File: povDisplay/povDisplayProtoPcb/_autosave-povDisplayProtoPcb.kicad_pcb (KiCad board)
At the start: 4 copper layers, 41 parts, among them J5 Conn_02x06_Odd_Even

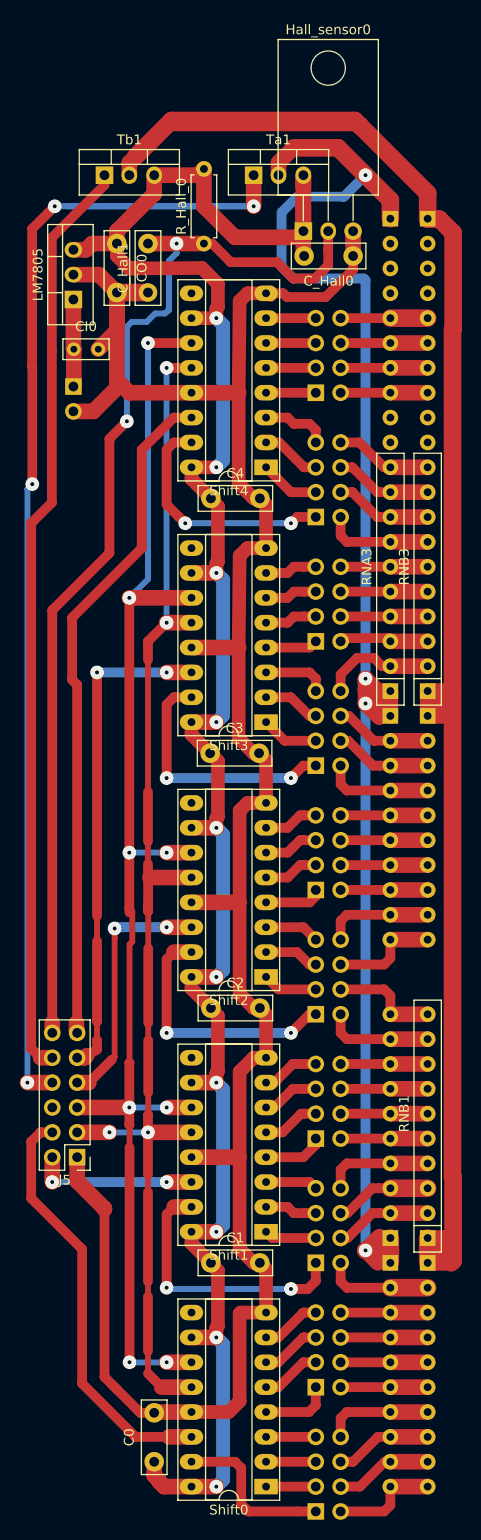
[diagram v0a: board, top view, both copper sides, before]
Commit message: Work on pcb.
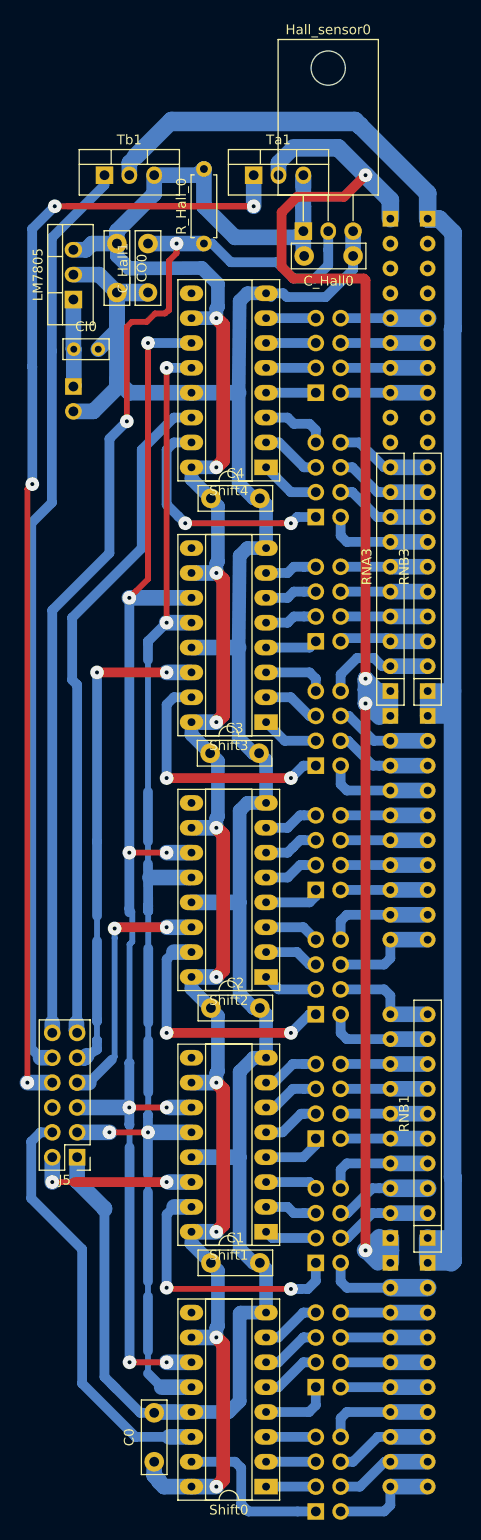
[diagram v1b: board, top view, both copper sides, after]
